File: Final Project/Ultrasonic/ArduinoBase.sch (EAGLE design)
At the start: 19 parts, among them IC1 ATTINY44-SSU, IC3 OPAMPSOT23-5

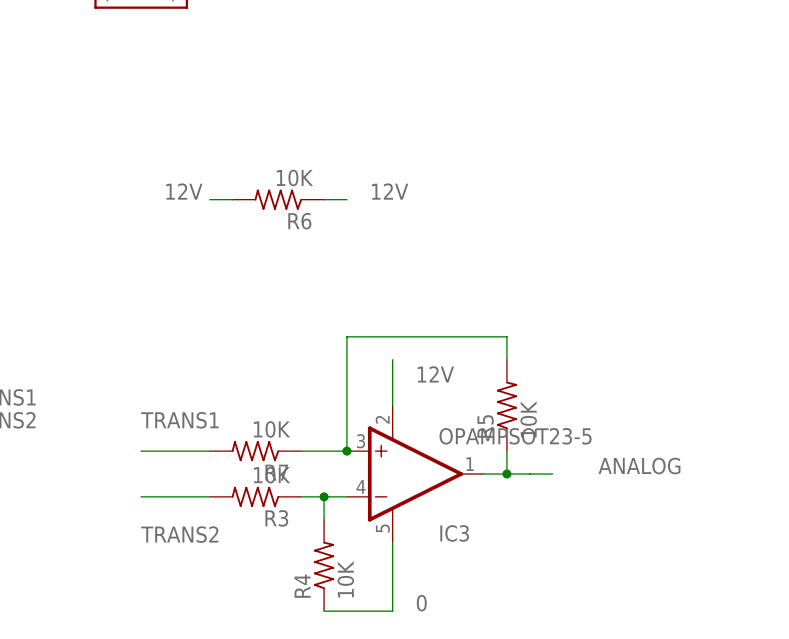
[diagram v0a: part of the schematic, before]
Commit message: Sensor ultrasonico
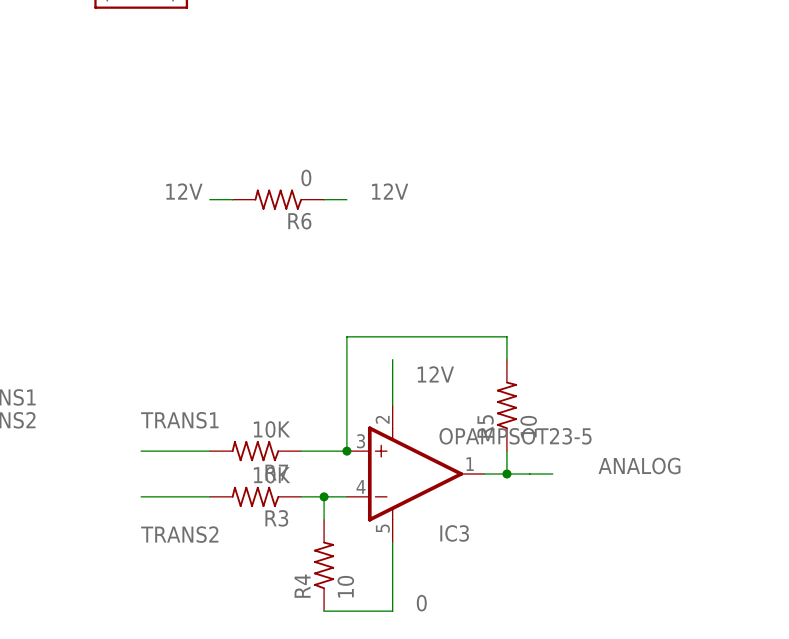
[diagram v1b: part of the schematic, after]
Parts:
- R4, R5: value 10K -> 10
- R6: value 10K -> 0
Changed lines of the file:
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@@
 <part name="U$6" library="fab" deviceset="PINHD-2X2-SMD" device=""/>
 <part name="R3" library="fab" deviceset="RES-US" device="1206FAB" value="10K"/>
-<part name="R4" library="fab" deviceset="RES-US" device="1206FAB" value="10K"/>
-<part name="R5" library="fab" deviceset="RES-US" device="1206FAB" value="10K"/>
-<part name="R6" library="fab" deviceset="RES-US" device="1206FAB" value="10K"/>
+<part name="R4" library="fab" deviceset="RES-US" device="1206FAB" value="10"/>
+<part name="R5" library="fab" deviceset="RES-US" device="1206FAB" value="10"/>
+<part name="R6" library="fab" deviceset="RES-US" device="1206FAB" value="0"/>
 <part name="R7" library="fab" deviceset="RES-US" device="1206FAB" value="10K"/>
 </parts>
